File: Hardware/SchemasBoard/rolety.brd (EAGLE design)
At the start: 49.9 x 22.9 mm, 30 parts, among them IC1 LNK304, IC2 MCP1703DB, K1 FRS1B, K2 FRS1B, T1 BC846, T2 BC846

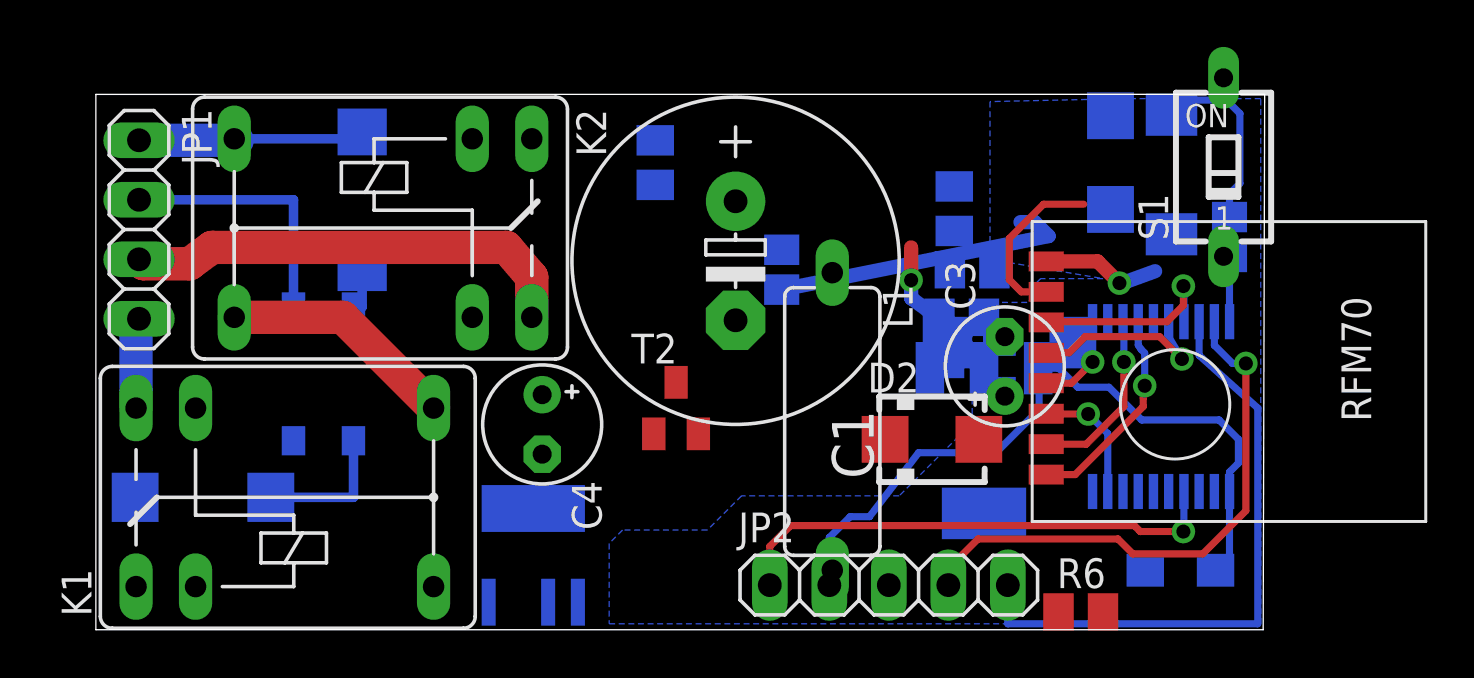
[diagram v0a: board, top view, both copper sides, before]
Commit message: aaa
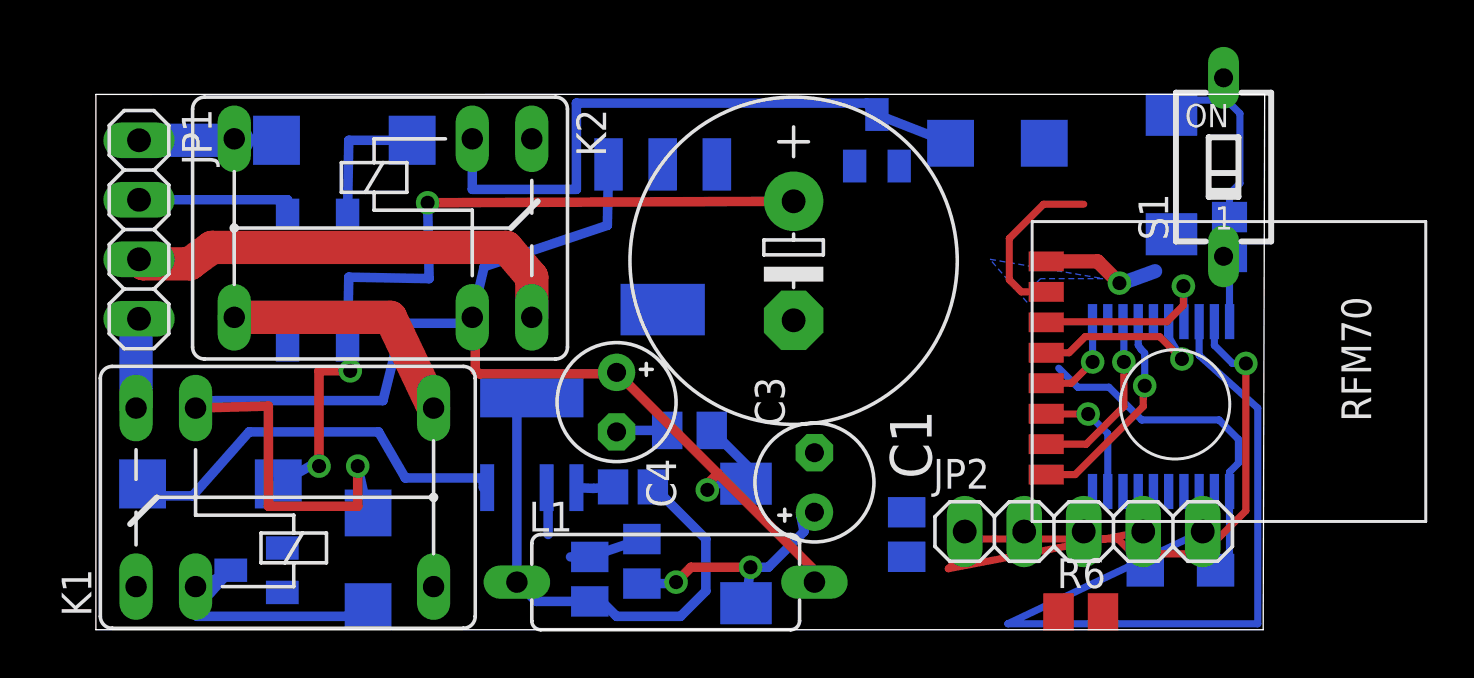
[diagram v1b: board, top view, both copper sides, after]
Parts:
- moved D1 35.9 mm to (11.6, 2.98)
- moved T1 31.8 mm to (6.86, 2.54)
- moved R3 18.8 mm to (23.3, 2.92), turned to 90 degrees
- moved R4 18.0 mm to (21.1, 2.16), turned to 270 degrees
- moved IC2 16.2 mm to (24.2, 16.8)
- moved T2 14.3 mm to (33.3, 20.9), flipped to the bottom
- moved D4 14.2 mm to (27.7, 3.68), turned to 90 degrees
- moved R5 14.1 mm to (34.6, 4.06)
- moved D2 12.9 mm to (38.5, 20.8), flipped to the bottom
- moved R7 12.6 mm to (25.3, 8.51), turned to 180 degrees
- moved C2 11.2 mm to (22.9, 6.10), turned to 180 degrees
- moved L1 9.88 mm to (24.3, 2.03), turned to 0 degrees
- moved C3 9.52 mm to (30.7, 6.29)
- moved JP2 8.63 mm to (42.2, 4.19)
- moved IC1 4.89 mm to (18.6, 8.06)
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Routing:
- net N$27: track 6.03 -> 66.4 mm, vias 1 -> 2
- net N$2: track 5.94 -> 33.6 mm, vias 0 -> 3
- net N$24: track 0.00 -> 26.7 mm
- net N$13: track 0.00 -> 22.8 mm
- net N$25: track 21.5 -> 0.00 mm, vias 1 -> 0
- net N$1: track 0.00 -> 18.3 mm
- net N$17: track 45.5 -> 29.4 mm
- net N$14: track 0.38 -> 12.9 mm
- net N$10: track 13.1 -> 1.57 mm
- net N$9: track 0.00 -> 10.8 mm, vias 0 -> 2
- net N$18: track 23.9 -> 31.7 mm
- net N$19: track 26.3 -> 33.9 mm
- net N$11: track 0.00 -> 5.20 mm
- net N$4: track 11.2 -> 6.91 mm
- net N$36: track 9.94 -> 6.00 mm
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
